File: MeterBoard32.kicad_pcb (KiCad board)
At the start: 2 copper layers, 49 x 63.3 mm, 38 parts, among them J1 Screw_Terminal_01x02, M1 MICRO_USB_18_TH, Q1 S8050, Q2 S8050, U1 AMS1117-3V3, U2 CP2102N-GQFN24, U3 ESP32-WROOM, U5 TSS721A

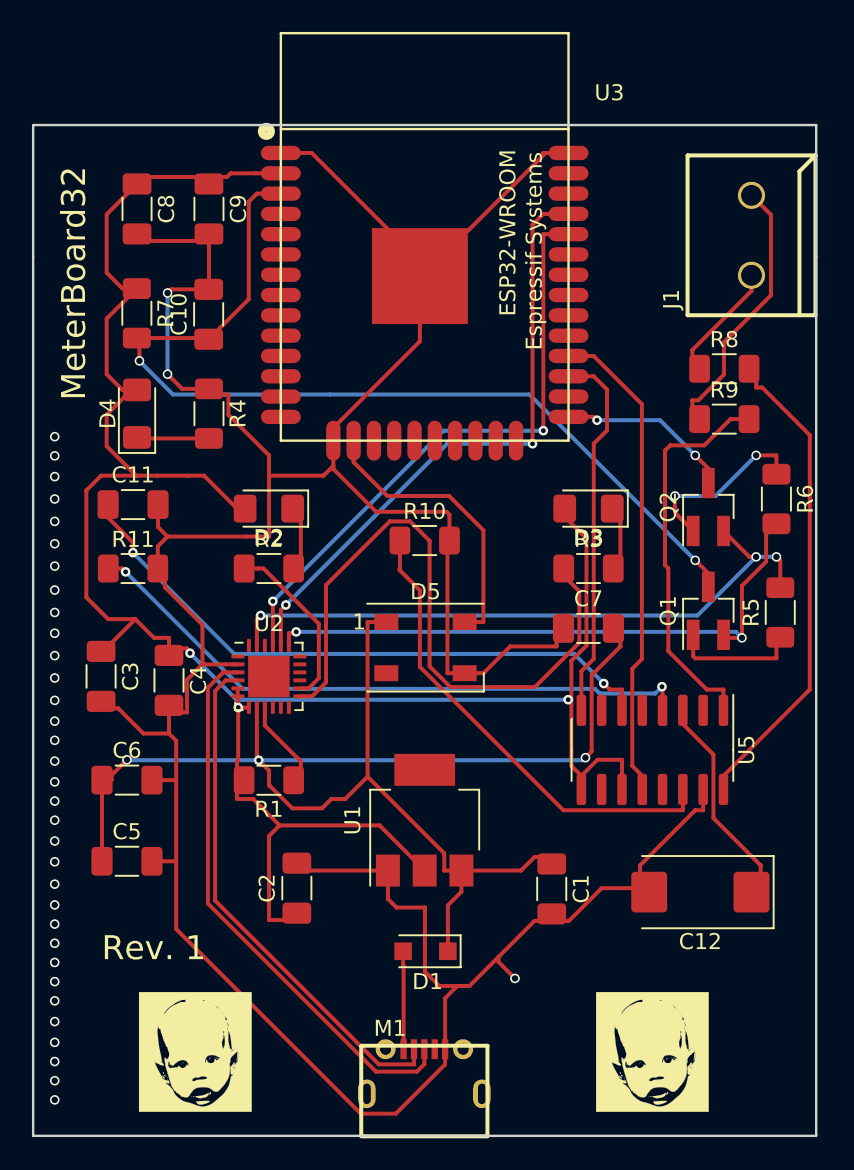
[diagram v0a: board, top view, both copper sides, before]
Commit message: Small fix
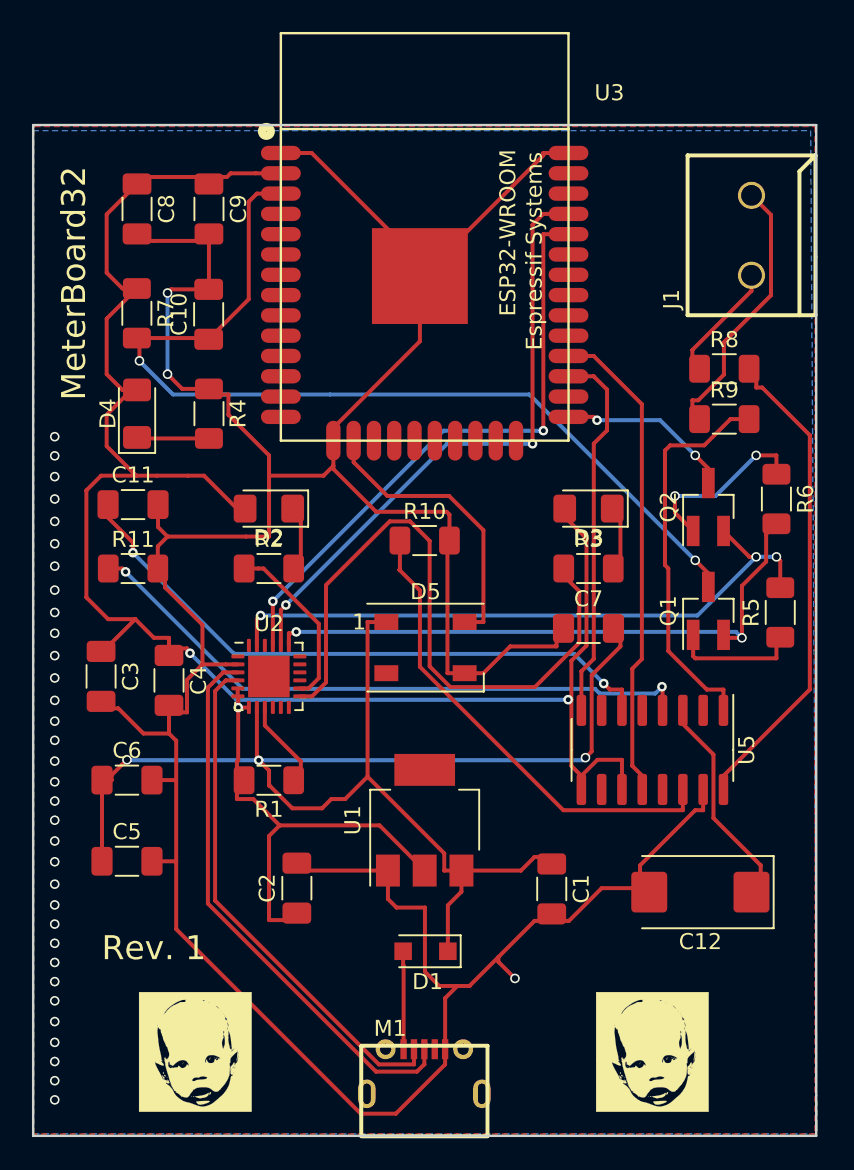
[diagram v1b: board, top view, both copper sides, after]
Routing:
- added copper zone on B.Cu, net GND
- added copper zone on F.Cu, net GND
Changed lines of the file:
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@@
   (via (at 108.1 84.8) (size 0.6) (drill 0.4) (layers F.Cu B.Cu) (net 2))
   (segment (start 107.06235 83.76235) (end 108.1 84.8) (width 0.25) (layer F.Cu) (net 2))
-  (segment (start 119.3744 74.2753) (end 115.925 77.7247) (width 0.25) (layer F.Cu) (net 2))
-  (segment (start 119.875 74.2753) (end 119.3744 74.2753) (width 0.25) (layer F.Cu) (net 2))
   (segment (start 119.875 73.2) (end 119.875 74.2753) (width 0.25) (layer F.Cu) (net 2))
   (segment (start 115.925 79.4) (end 115.925 79.15) (width 0.25) (layer F.Cu) (net 2))
@@
   (segment (start 102.15 44.935) (end 102.15 41.196) (width 0.25) (layer F.Cu) (net 2))
   (segment (start 96.735 51.15) (end 96.735 50.35) (width 0.25) (layer F.Cu) (net 2))
+  (segment (start 119.3744 74.2753) (end 115.925 77.7247) (width 0.25) (layer F.Cu) (net 2))
+  (segment (start 119.875 74.2753) (end 119.3744 74.2753) (width 0.25) (layer F.Cu) (net 2))
   (segment (start 84.1625 48.26) (end 84.45 47.9725) (width 0.25) (layer F.Cu) (net 3))
   (segment (start 84.45 47.9725) (end 83.5325 47.9725) (width 0.25) (layer F.Cu) (net 3))
@@
   (via (at 118.11 54.60999) (size 0.6) (drill 0.4) (layers F.Cu B.Cu) (net 75))
   (segment (start 123.19 52.07) (end 120.65001 54.60999) (width 0.25) (layer B.Cu) (net 75))
+  (zone (net 2) (net_name GND) (layer F.Cu) (hatch edge 0.508)
+    (connect_pads (clearance 0.508))
+    (min_thickness 0.254)
+    (fill yes (arc_segments 32) (thermal_gap 0.508) (thermal_bridge_width 0.508))
+    (polygon
+      (pts
+        (xy 126.86873 94.534859) (xy 77.98975 94.534859) (xy 77.98975 31.543983) (xy 78.039746 31.493987) (xy 126.86873 31.493987)
+      )
+    )
+    (polygon
+      (pts
+        (xy 78.039746 31.493987) (xy 77.989877 31.493987) (xy 78.013218 31.517328) (xy 77.98975 31.517328) (xy 77.98975 31.493987)
+        (xy 77.989877 31.493987) (xy 77.98975 31.49386) (xy 78.039873 31.49386)
+      )
+    )
+  )
+  (zone (net 2) (net_name GND) (layer B.Cu) (hatch edge 0.508)
+    (connect_pads (clearance 0.508))
+    (min_thickness 0.254)
+    (fill yes (arc_segments 32) (thermal_gap 0.508) (thermal_bridge_width 0.508))
+    (polygon
+      (pts
+        (xy 127 93.98) (xy 127 94.531007) (xy 77.940469 94.531007) (xy 77.940469 31.75) (xy 126.602539 31.75)
+      )
+    )
+  )
 )
